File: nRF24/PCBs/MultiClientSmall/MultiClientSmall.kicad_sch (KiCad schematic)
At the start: 12 parts, among them M1 TP4056, SW1 SW_Push_Dual, U1 NRF24L01, U2 ATtiny84, U3 MCP1700x-330, U4 BH1750, U5 AM312

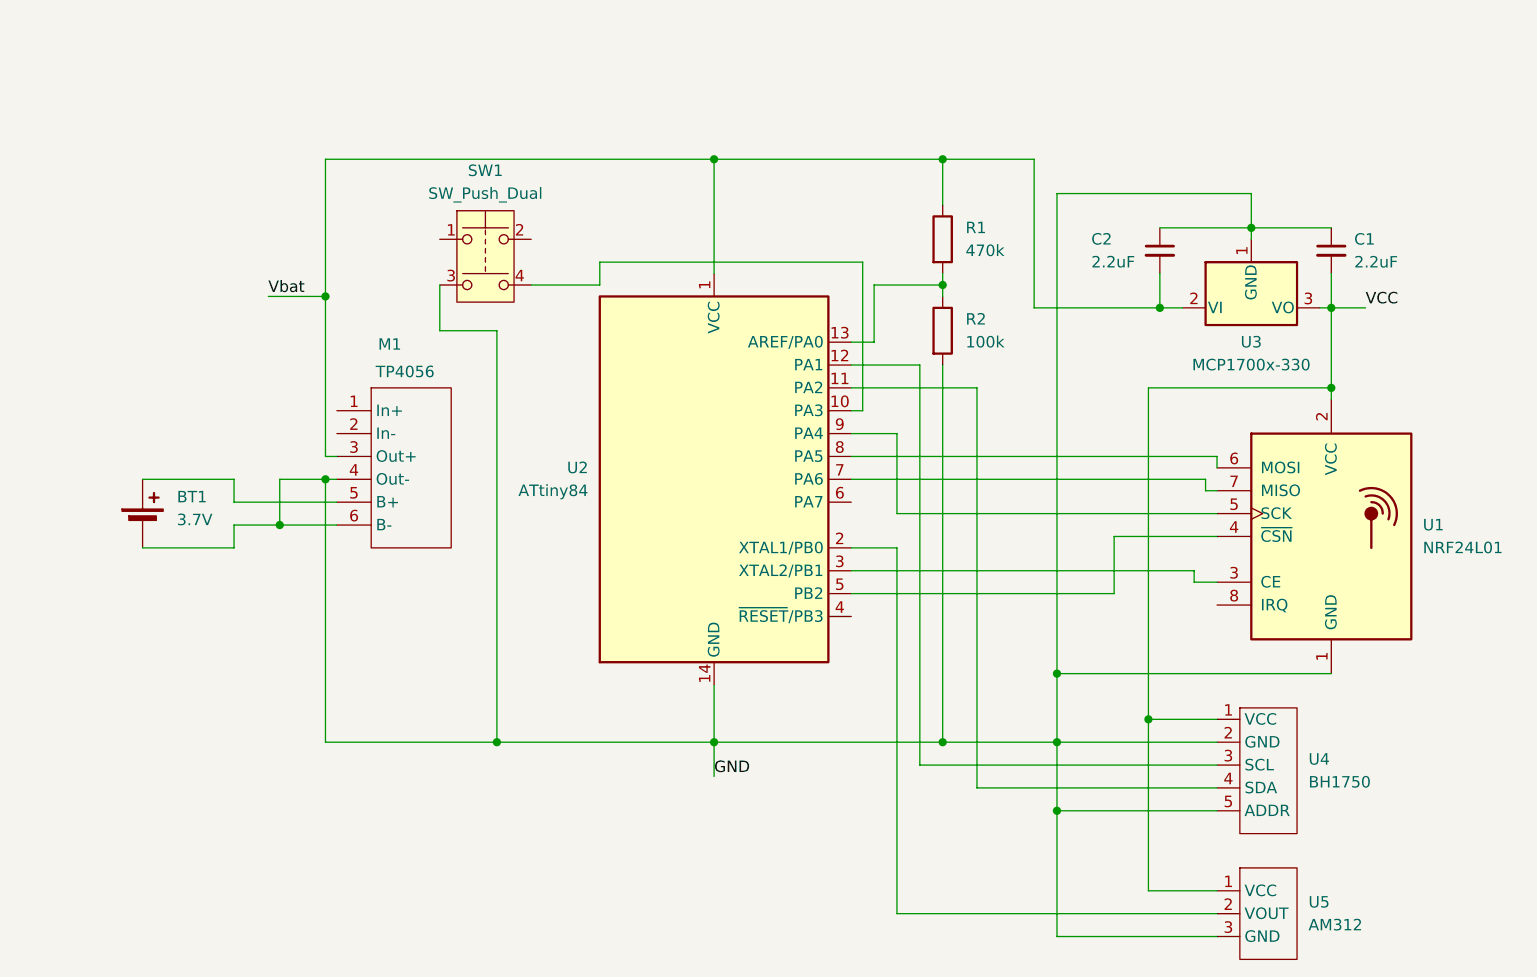
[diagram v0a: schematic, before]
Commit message: Production Version of nRF24 Multi Client Small
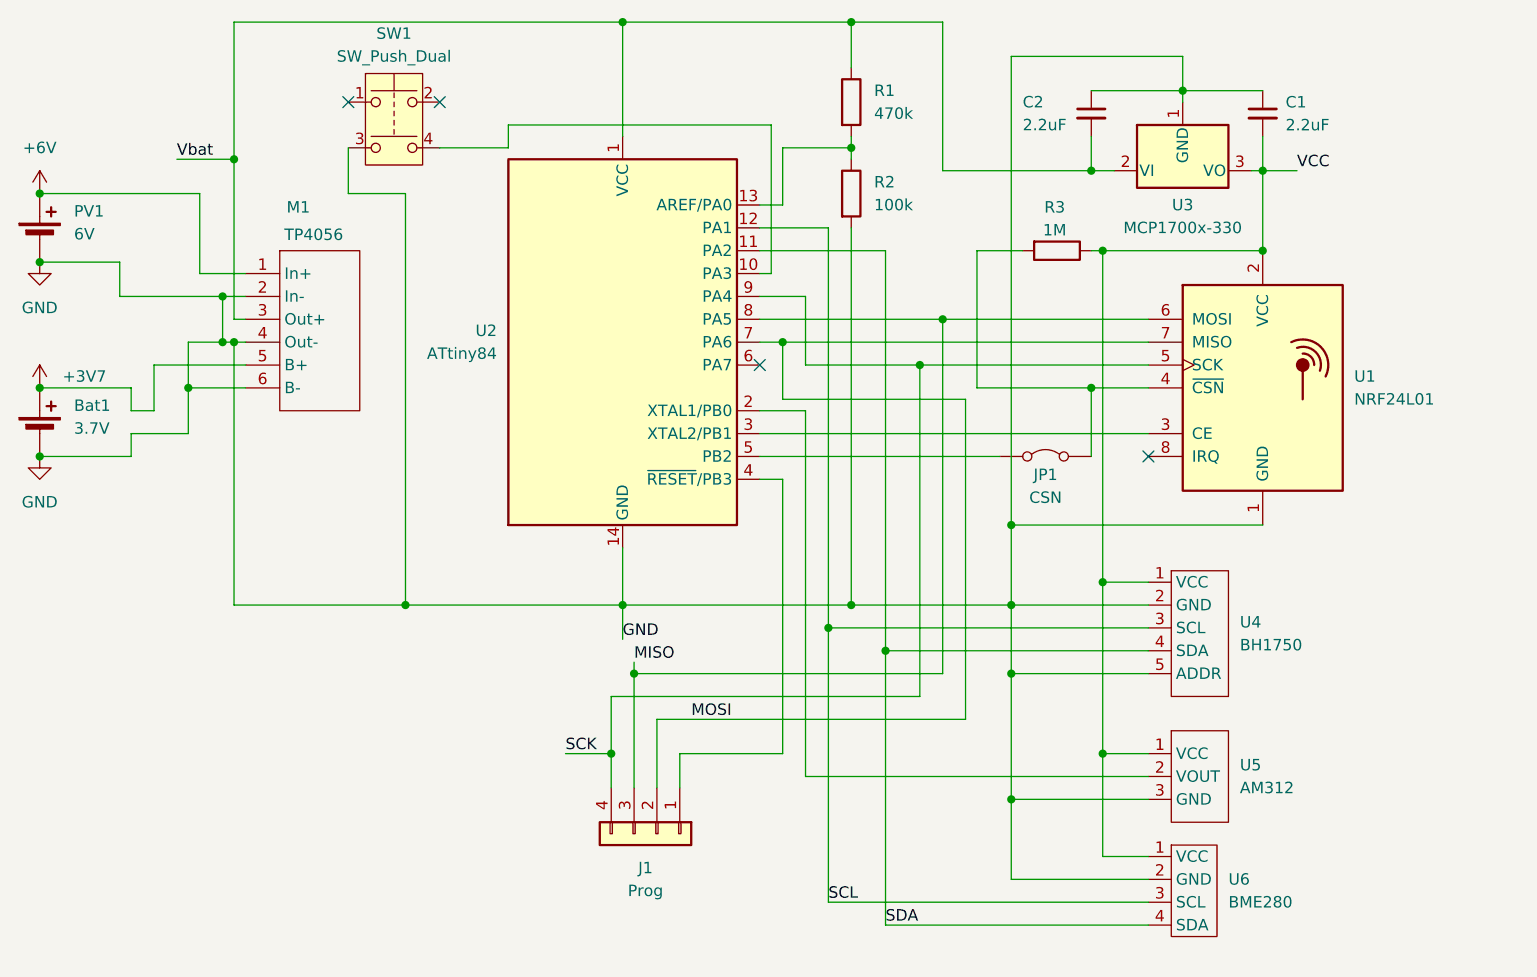
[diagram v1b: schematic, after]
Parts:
- added J1: Prog, Connector_PinHeader_2.54mm:PinHeader_1x04_P2.54mm_Vertical, symbol Connector_Generic:Conn_01x04
- added JP1: CSN, Connector_PinHeader_2.54mm:PinHeader_1x02_P2.54mm_Vertical, symbol Jumper:Jumper_2_Bridged
- added PV1: 6V, hagego:JST_PH_1x02_P2.00, symbol Device:Battery_Cell
- added R3: 1M, Resistor_THT:R_Axial_DIN0207_L6.3mm_D2.5mm_P10.16mm_Horizontal, symbol Device:R
- added U6: BME280, hagego:BME280, symbol hagego:BME280_Module
- Bat1: renamed from BT1; footprint Connector_JST:JST_PH_B2B-PH-K_1x02_P2.00mm_Vertical -> hagego:JST_PH_1x02_P2.00
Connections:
- net GND: now also M1.2 (In-), PV1.2 (-), U6.2 (GND)
- net VCC: now also R3.1, U6.1 (VCC)
- net at U1.4 (~{CSN}): now also JP1.2 (B), R3.2; no longer U2.5 (PB2)
- net SCK: now reaches U1.5 (SCK), U2.9 (PA4)
- net SCK: now also J1.4 (Pin_4)
- net MISO: now reaches U1.6 (MOSI), U2.8 (PA5)
- net MISO: now also J1.3 (Pin_3)
- net MOSI: now reaches U1.7 (MISO), U2.7 (PA6)
- net MOSI: now also J1.2 (Pin_2)
- net SDA: now reaches U2.11 (PA2), U4.4 (SDA)
- net SDA: now also U6.4 (SDA)
- net SCL: now reaches U2.12 (PA1), U4.3 (SCL)
- net SCL: now also U6.3 (SCL)
- net at U2.4 (~{RESET}/PB3): now also J1.1 (Pin_1)
- net +3V7: now reaches Bat1.1 (+), M1.5 (B+)
- net +6V: now reaches M1.1 (In+)
- net +6V: now also PV1.1 (+)
- new net: JP1.1 (A), U2.5 (PB2)
- no-connect marks 0 -> 4
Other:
- title: nRF24 Button -> nRF24 Multi Client
- moved on the sheet: Bat1, C1, C2, M1, R1, R2, SW1, U1, U2, U3, U4, U5
